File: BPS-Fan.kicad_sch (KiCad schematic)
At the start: 37 parts, among them J1 LDRBRDConn, J10 FAN9, J11 FAN10, J12 FAN11, J13 FAN12, J2 FAN1, J3 FAN2, J4 FAN3, J5 FAN4, J6 FAN5, J7 FAN6, J8 FAN7, J9 FAN8, Q1 BUK9M23-80E, Q2 BUK9M23-80E, Q3 BUK9M23-80E, Q4 BUK9M23-80E

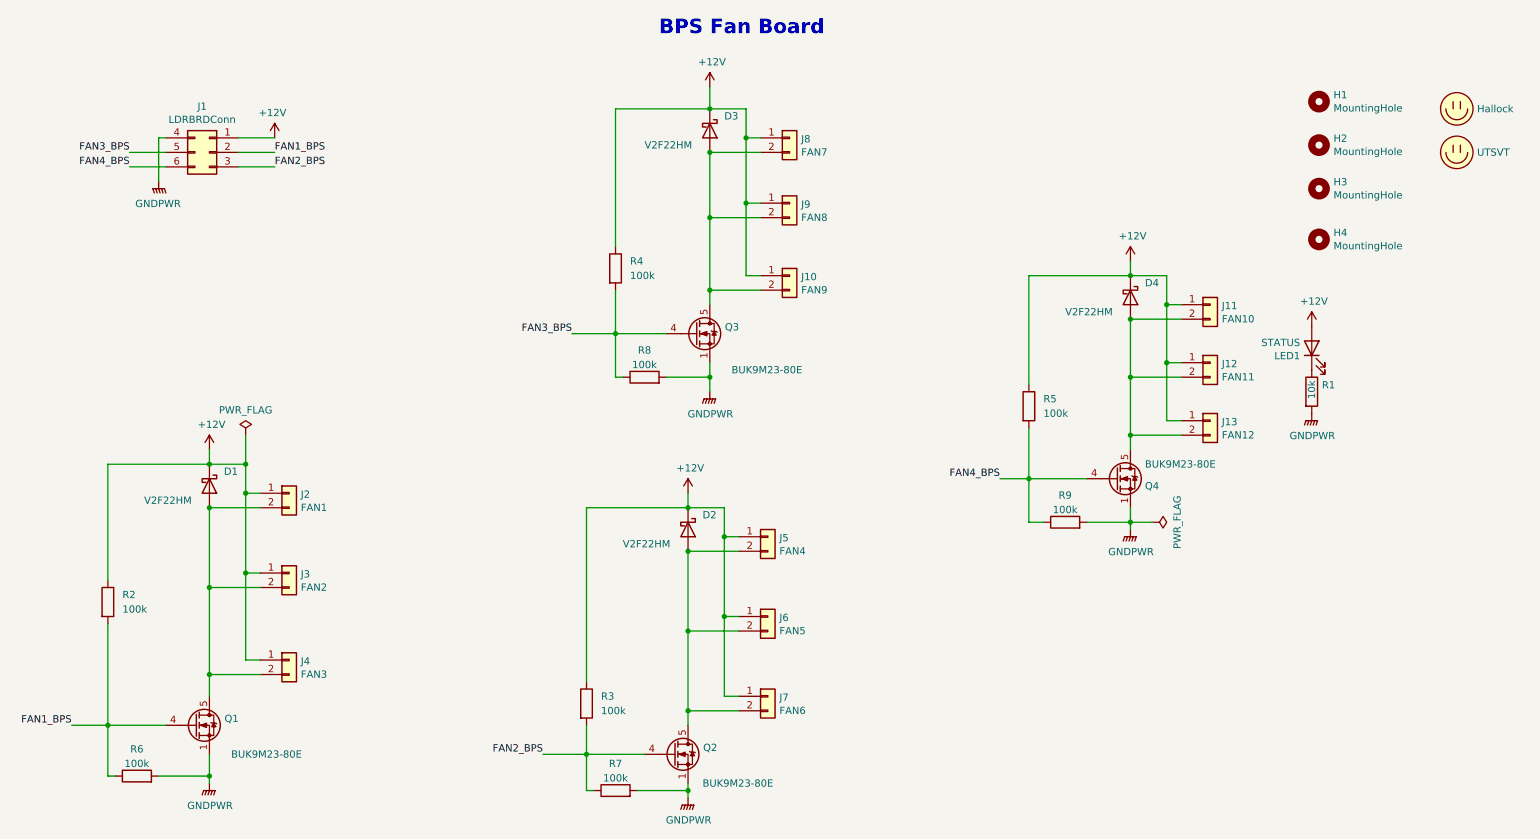
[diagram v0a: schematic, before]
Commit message: fan go brrr
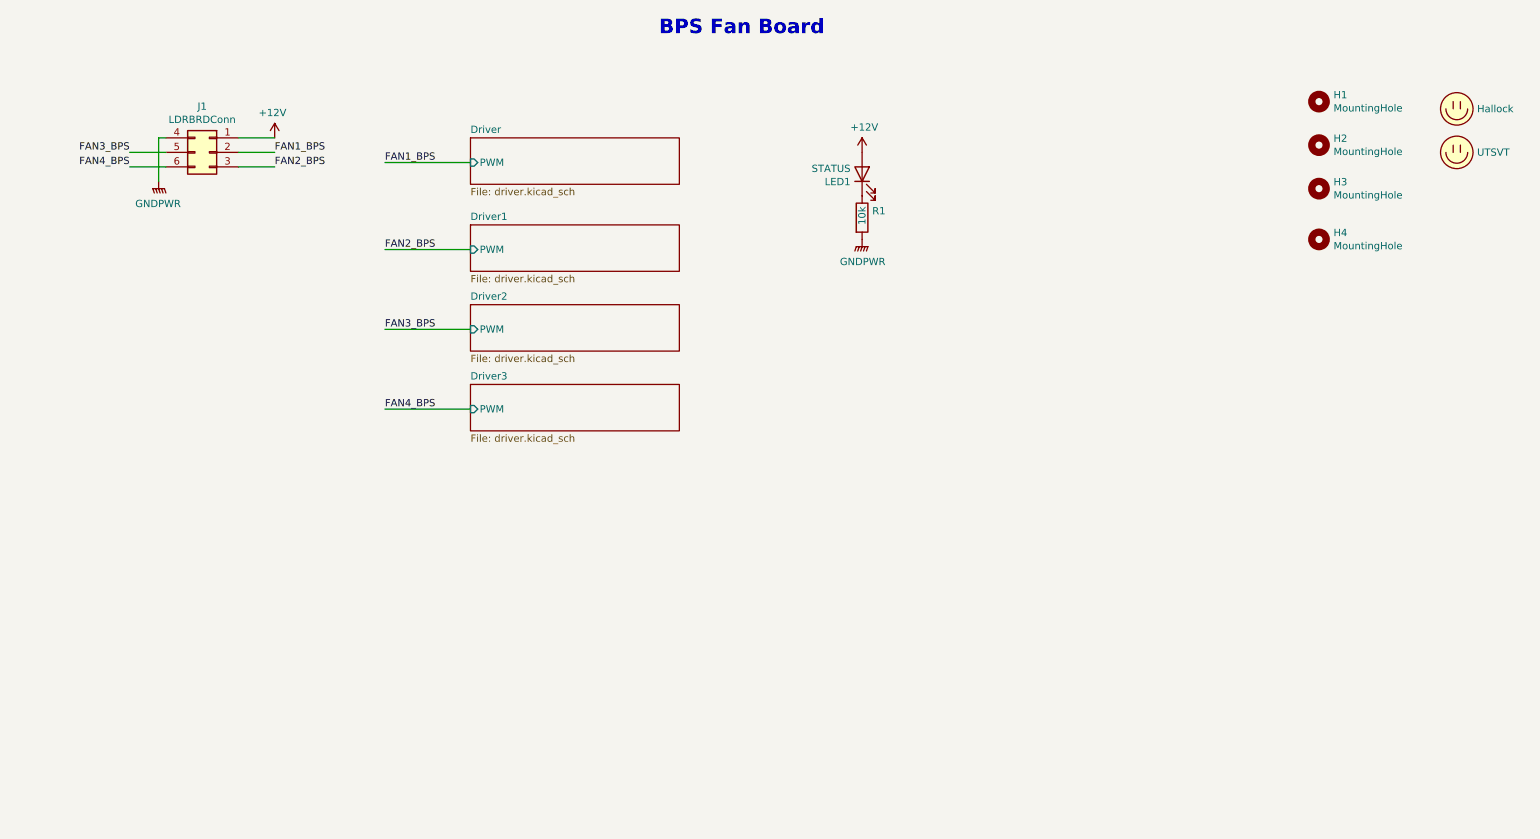
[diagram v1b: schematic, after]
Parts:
- removed D1, D2, D3, D4: V2F22HM, UTSVT_Passive:V2F22HM, symbol Diode:C3D25170H
- removed J10: FAN9, UTSVT_Connectors:Molex_MicroFit3.0_1x2xP3.00mm_PolarizingPeg_Vertical, symbol Connector_Generic:Conn_01x02
- removed J11: FAN10, UTSVT_Connectors:Molex_MicroFit3.0_1x2xP3.00mm_PolarizingPeg_Vertical, symbol Connector_Generic:Conn_01x02
- removed J12: FAN11, UTSVT_Connectors:Molex_MicroFit3.0_1x2xP3.00mm_PolarizingPeg_Vertical, symbol Connector_Generic:Conn_01x02
- removed J13: FAN12, UTSVT_Connectors:Molex_MicroFit3.0_1x2xP3.00mm_PolarizingPeg_Vertical, symbol Connector_Generic:Conn_01x02
- removed J2: FAN1, UTSVT_Connectors:Molex_MicroFit3.0_1x2xP3.00mm_PolarizingPeg_Vertical, symbol Connector_Generic:Conn_01x02
- removed J3: FAN2, UTSVT_Connectors:Molex_MicroFit3.0_1x2xP3.00mm_PolarizingPeg_Vertical, symbol Connector_Generic:Conn_01x02
- removed J4: FAN3, UTSVT_Connectors:Molex_MicroFit3.0_1x2xP3.00mm_PolarizingPeg_Vertical, symbol Connector_Generic:Conn_01x02
- removed J5: FAN4, UTSVT_Connectors:Molex_MicroFit3.0_1x2xP3.00mm_PolarizingPeg_Vertical, symbol Connector_Generic:Conn_01x02
- removed J6: FAN5, UTSVT_Connectors:Molex_MicroFit3.0_1x2xP3.00mm_PolarizingPeg_Vertical, symbol Connector_Generic:Conn_01x02
- removed J7: FAN6, UTSVT_Connectors:Molex_MicroFit3.0_1x2xP3.00mm_PolarizingPeg_Vertical, symbol Connector_Generic:Conn_01x02
- removed J8: FAN7, UTSVT_Connectors:Molex_MicroFit3.0_1x2xP3.00mm_PolarizingPeg_Vertical, symbol Connector_Generic:Conn_01x02
- removed J9: FAN8, UTSVT_Connectors:Molex_MicroFit3.0_1x2xP3.00mm_PolarizingPeg_Vertical, symbol Connector_Generic:Conn_01x02
- removed Q1, Q2, Q3, Q4: BUK9M23-80E, Package_TO_SOT_SMD:LFPAK33, symbol Transistor_FET:BUK9M23-80EX
- removed R2, R3, R4, R5, R6, R7, R8, R9: 100k, Resistor_SMD:R_0805_2012Metric, symbol Device:R
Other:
- added sheet Driver (driver.kicad_sch)
- added sheet Driver1 (driver.kicad_sch)
- added sheet Driver2 (driver.kicad_sch)
- added sheet Driver3 (driver.kicad_sch)
- moved on the sheet: LED1, R1
